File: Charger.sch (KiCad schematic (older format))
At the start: 43 parts, among them J1 Input, J2 USB-A-S-X-X-SM2, J3 USB-A-S-X-X-SM2, Q1 BSC42DN25NS3, T1 760875131, U1 LT1085-5.0, U2 TPS2546, U3 LT3798MPMSETRPBF, U4 TPS2546RTER

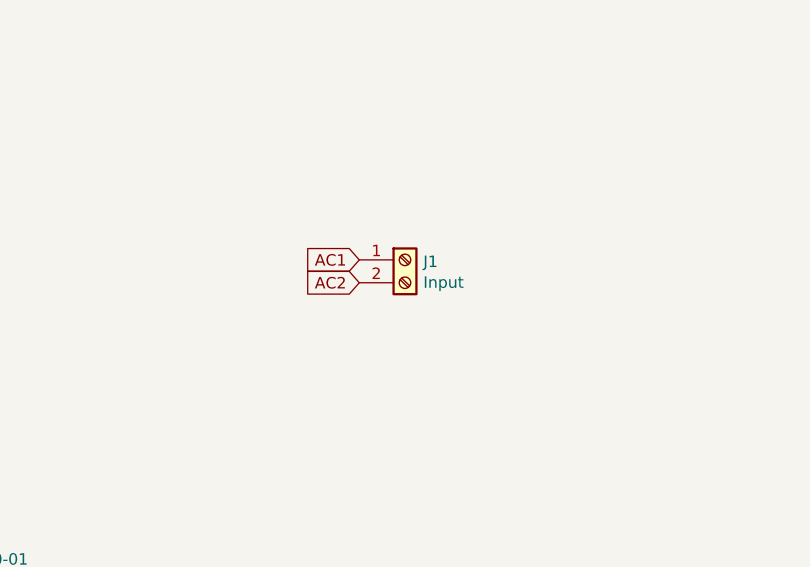
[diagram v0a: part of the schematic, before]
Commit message: compact
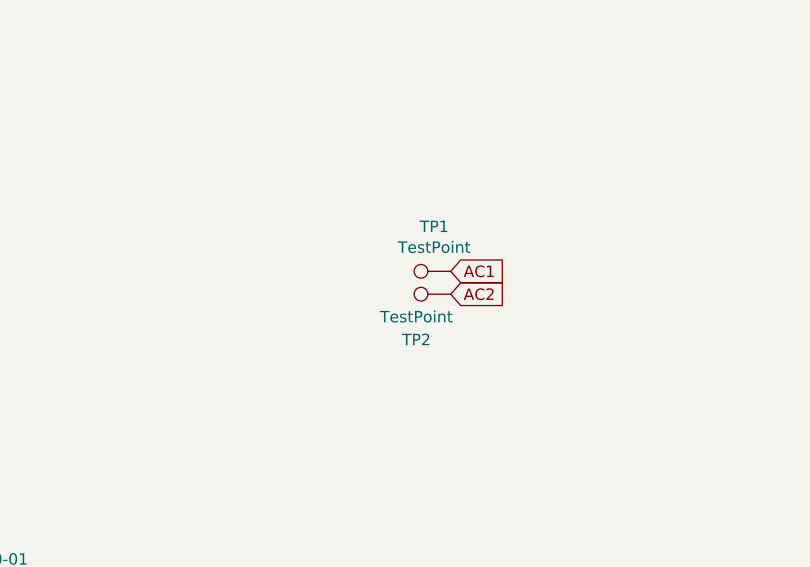
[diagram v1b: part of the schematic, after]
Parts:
- removed J1: Input, TerminalBlock:TerminalBlock_bornier-2_P5.08mm, symbol Connector:Screw_Terminal_01x02
- added TP1, TP2: TestPoint, TestPoint:TestPoint_Pad_2.0x2.0mm, symbol Connector:TestPoint
- C1: footprint Capacitor_THT:CP_Radial_D10.0mm_P7.50mm -> Capacitor_SMD:CP_Elec_5x4.4
- C3: footprint Capacitor_SMD:CP_Elec_3x5.3 -> Capacitor_SMD:CP_Elec_4x3.9
- C4, C5, C7, C9: footprint Capacitor_THT:CP_Radial_D4.0mm_P1.50mm -> Capacitor_SMD:CP_Elec_3x5.3
- C8: footprint Capacitor_THT:CP_Radial_D8.0mm_P3.80mm -> Capacitor_SMD:CP_Elec_5x4.4
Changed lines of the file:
@@
 F 0 "C3" H 6778 3296 50  0000 L CNN
 F 1 "47u" H 6778 3205 50  0000 L CNN
-F 2 "Capacitor_SMD:CP_Elec_3x5.3" H 6600 3250 50  0001 C CNN
+F 2 "Capacitor_SMD:CP_Elec_4x3.9" H 6600 3250 50  0001 C CNN
 F 3 "~" H 6600 3250 50  0001 C CNN
 	1    6600 3250
-	1    0    0    -1
-$EndComp
-$Comp
-L Connector:Screw_Terminal_01x02 J1
-U 1 1 6031590C
-P 3600 700
-F 0 "J1" H 3680 692 50  0000 L CNN
-F 1 "Input" H 3680 601 50  0000 L CNN
-F 2 "TerminalBlock:TerminalBlock_bornier-2_P5.08mm" H 3600 700 50  0001 C CNN
-F 3 "~" H 3600 700 50  0001 C CNN
-	1    3600 700
 	1    0    0    -1
 $EndComp
@@
 NoConn ~ 7250 3250
 NoConn ~ 8650 3850
-Text GLabel 3400 700  0    50   Input ~ 0
+Text GLabel 3800 750  2    50   Input ~ 0
 AC1
-Text GLabel 3400 800  0    50   Input ~ 0
+Text GLabel 3800 850  2    50   Input ~ 0
 AC2
 Wire Wire Line
@@
 F 0 "C4" H 1928 7196 50  0000 L CNN
 F 1 "0.1u" H 1928 7105 50  0000 L CNN
-F 2 "Capacitor_THT:CP_Radial_D4.0mm_P1.50mm" H 1750 7150 50  0001 C CNN
+F 2 "Capacitor_SMD:CP_Elec_3x5.3" H 1750 7150 50  0001 C CNN
 F 3 "~" H 1750 7150 50  0001 C CNN
 	1    1750 7150
@@
 F 0 "C9" H 6115 7346 50  0000 L CNN
 F 1 "22p" H 6115 7255 50  0000 L CNN
-F 2 "Capacitor_THT:CP_Radial_D4.0mm_P1.50mm" H 6038 7150 50  0001 C CNN
+F 2 "Capacitor_SMD:CP_Elec_3x5.3" H 6038 7150 50  0001 C CNN
 F 3 "~" H 6000 7300 50  0001 C CNN
 	1    6000 7300
@@
 F 0 "C1" H 2115 2396 50  0000 L CNN
 F 1 "470u" H 2115 2305 50  0000 L CNN
-F 2 "Capacitor_THT:CP_Radial_D10.0mm_P7.50mm" H 2038 2200 50  0001 C CNN
+F 2 "Capacitor_SMD:CP_Elec_5x4.4" H 2038 2200 50  0001 C CNN
 F 3 "~" H 2000 2350 50  0001 C CNN
 	1    2000 2350
@@
 F 0 "C5" H 2315 3346 50  0000 L CNN
 F 1 "10u" H 2315 3255 50  0000 L CNN
-F 2 "Capacitor_THT:CP_Radial_D4.0mm_P1.50mm" H 2238 3150 50  0001 C CNN
+F 2 "Capacitor_SMD:CP_Elec_3x5.3" H 2238 3150 50  0001 C CNN
 F 3 "~" H 2200 3300 50  0001 C CNN
 	1    2200 3300
@@
 F 0 "C7" V 4948 6950 50  0000 C CNN
 F 1 "4.7p" V 5039 6950 50  0000 C CNN
-F 2 "Capacitor_THT:CP_Radial_D4.0mm_P1.50mm" H 5238 6800 50  0001 C CNN
+F 2 "Capacitor_SMD:CP_Elec_3x5.3" H 5238 6800 50  0001 C CNN
 F 3 "~" H 5200 6950 50  0001 C CNN
 	1    5200 6950
@@
 F 0 "C8" H 6065 2896 50  0000 L CNN
 F 1 "470u" H 6065 2805 50  0000 L CNN
-F 2 "Capacitor_THT:CP_Radial_D8.0mm_P3.80mm" H 5988 2700 50  0001 C CNN
+F 2 "Capacitor_SMD:CP_Elec_5x4.4" H 5988 2700 50  0001 C CNN
 F 3 "~" H 5950 2850 50  0001 C CNN
 	1    5950 2850
@@
 	1    0    0    -1
 $EndComp
+$Comp
+L Connector:TestPoint TP1
+U 1 1 603D66F1
+P 3800 750
+F 0 "TP1" V 3995 822 50  0000 C CNN
+F 1 "TestPoint" V 3904 822 50  0000 C CNN
+F 2 "TestPoint:TestPoint_Pad_2.0x2.0mm" H 4000 750 50  0001 C CNN
+F 3 "~" H 4000 750 50  0001 C CNN
+	1    3800 750
+	0    -1   -1   0
+$EndComp
+$Comp
+L Connector:TestPoint TP2
+U 1 1 603D7132
+P 3800 850
+F 0 "TP2" V 3600 1000 50  0000 C CNN
+F 1 "TestPoint" V 3700 1000 50  0000 C CNN
+F 2 "TestPoint:TestPoint_Pad_2.0x2.0mm" H 4000 850 50  0001 C CNN
+F 3 "~" H 4000 850 50  0001 C CNN
+	1    3800 850
+	0    -1   -1   0
+$EndComp
 $EndSCHEMATC
